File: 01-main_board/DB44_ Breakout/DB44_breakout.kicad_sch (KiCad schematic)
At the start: 7 parts, among them J1 DB44_Female, J2 Screw_Terminal_01x10 (5.08 mm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, J3 Screw_Terminal_01x10, J4 Screw_Terminal_01x10, J5 Screw_Terminal_01x10, J6 Screw_Terminal_01x02, J7 Screw_Terminal_01x02

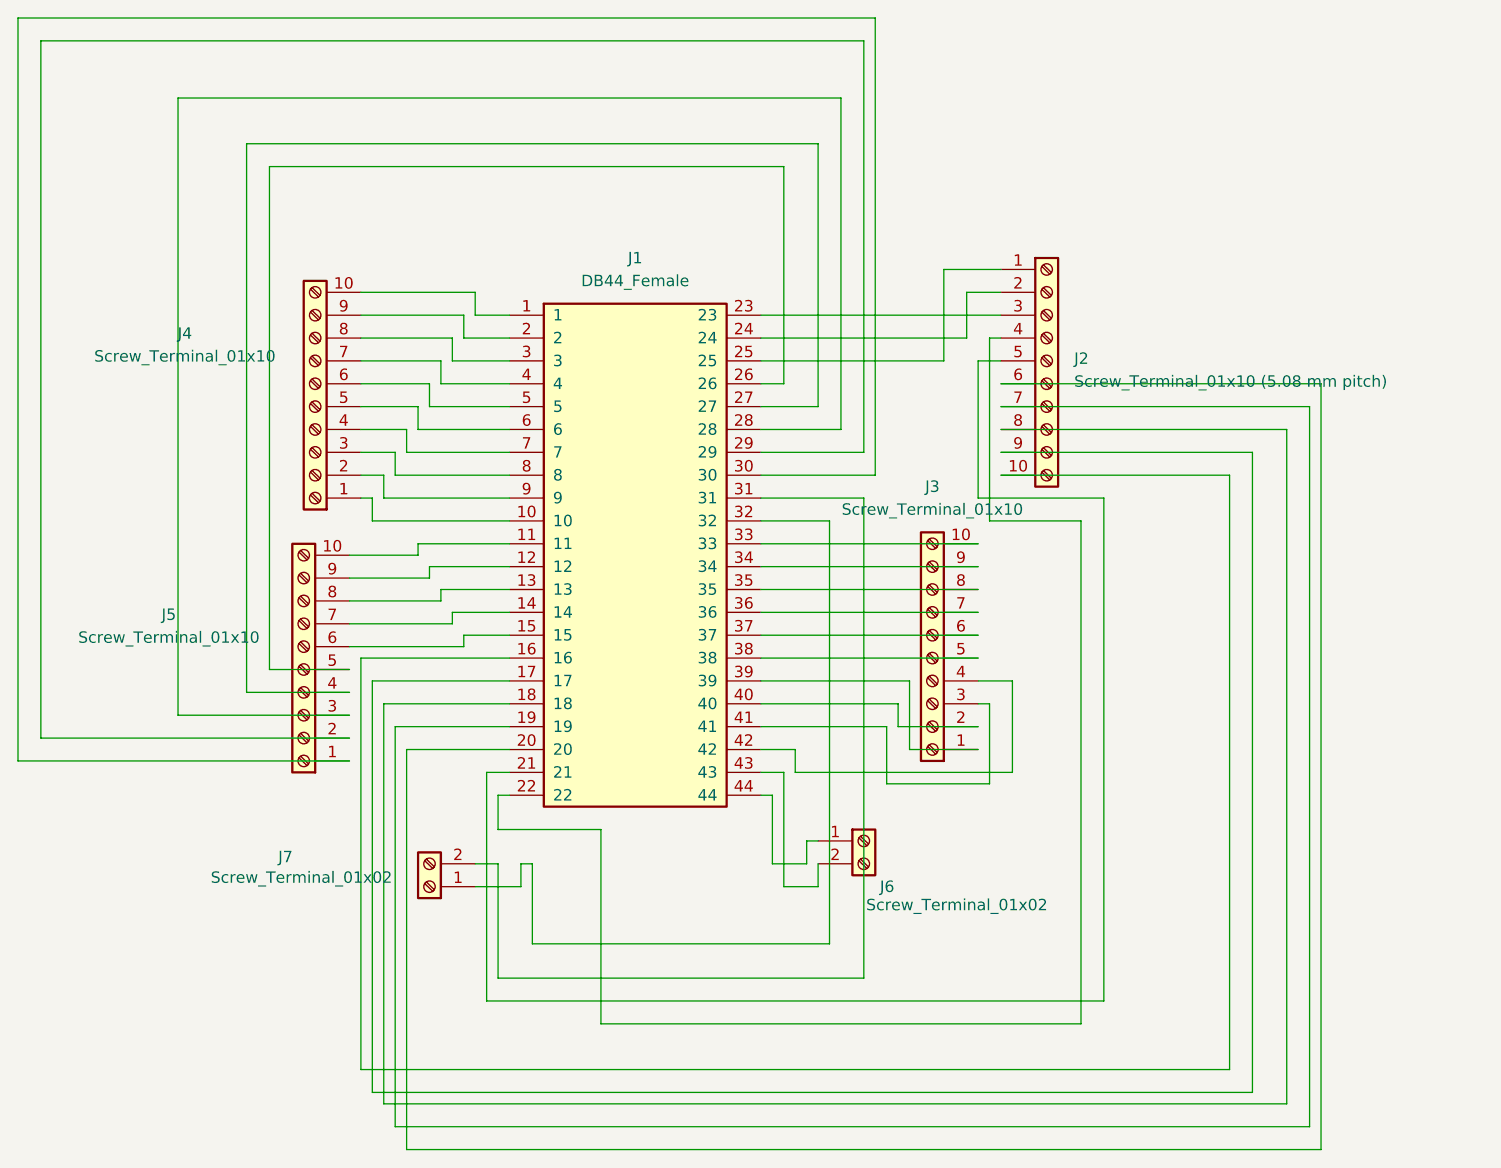
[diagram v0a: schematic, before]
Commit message: Finished DB44 board edits
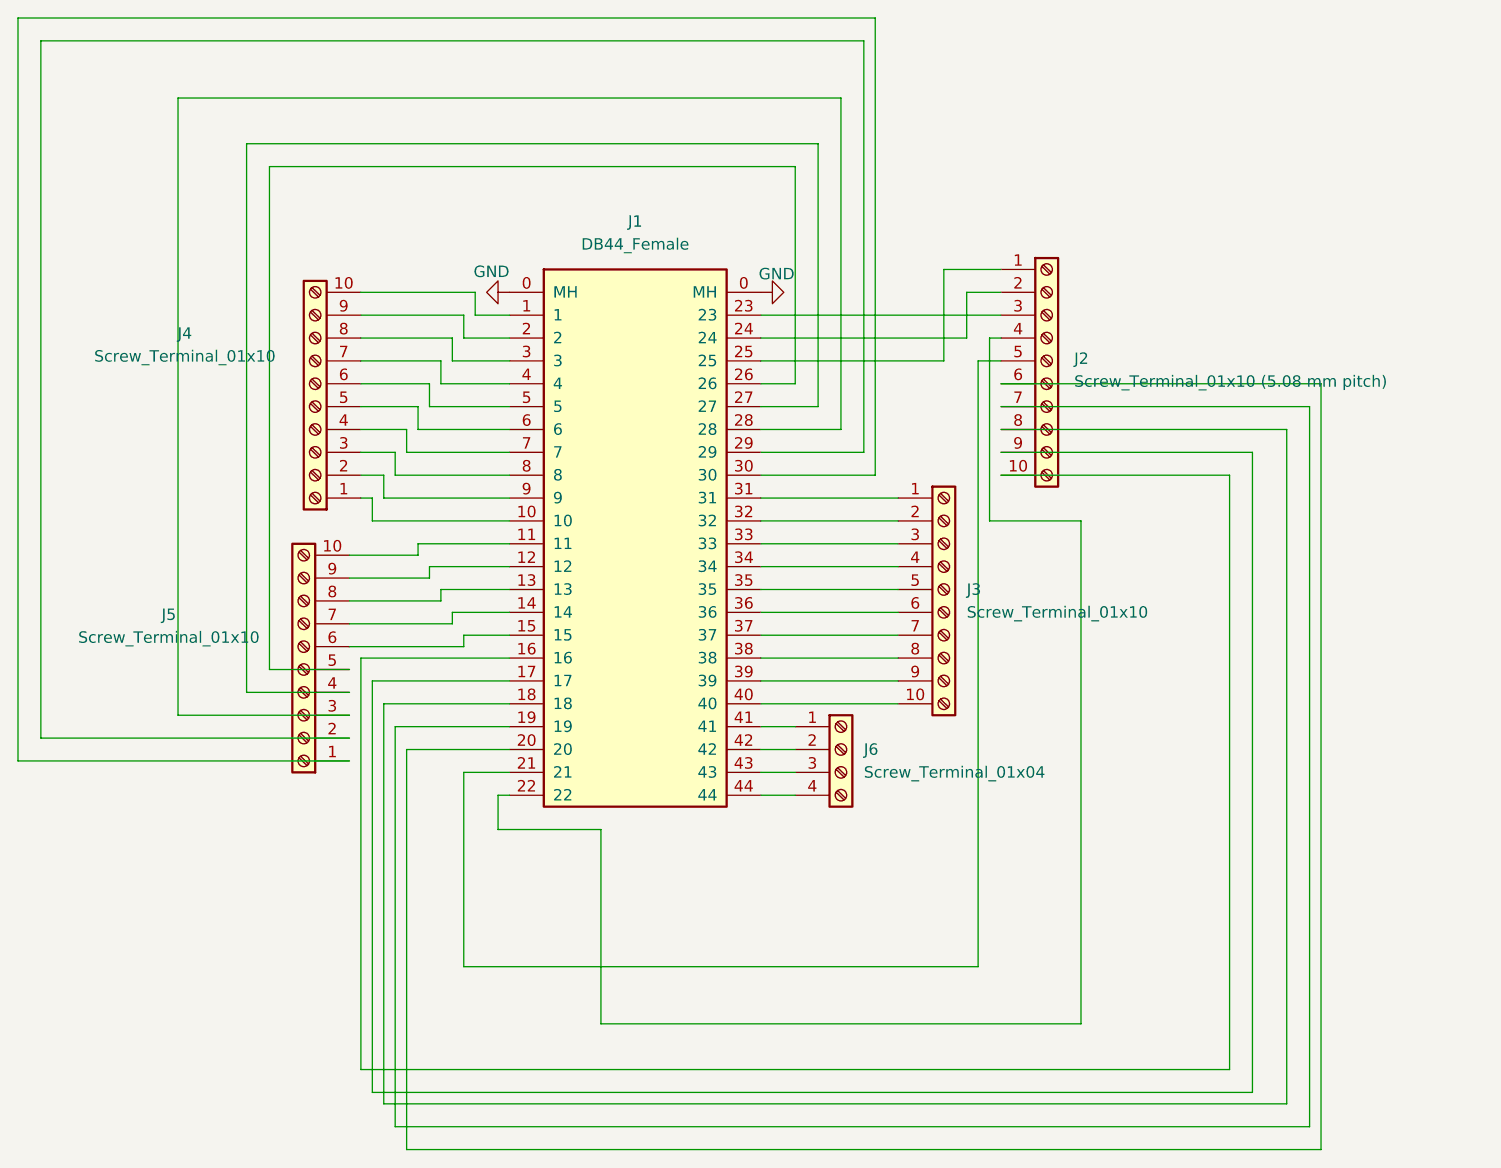
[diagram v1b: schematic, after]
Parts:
- removed J6, J7: Screw_Terminal_01x02, TerminalBlock_RND:TerminalBlock_RND_205-00232_1x02_P5.08mm_Horizontal, symbol Connector:Screw_Terminal_01x02
- added J6: Screw_Terminal_01x04, TerminalBlock_RND:TerminalBlock_RND_205-00234_1x04_P5.08mm_Horizontal, symbol Connector:Screw_Terminal_01x04
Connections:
- net at J3.1 (Pin_1): now also J1.31; no longer J1.39
- net at J3.10 (Pin_10): now also J1.40; no longer J1.33
- net at J3.2 (Pin_2): now also J1.32; no longer J1.40
- net at J3.3 (Pin_3): now also J1.33; no longer J1.41
- net at J3.4 (Pin_4): now also J1.34; no longer J1.42
- net at J3.5 (Pin_5): now also J1.35; no longer J1.38
- net at J3.6 (Pin_6): now also J1.36; no longer J1.37
- net at J3.7 (Pin_7): now also J1.37; no longer J1.36
- net at J3.8 (Pin_8): now also J1.38; no longer J1.35
- net at J3.9 (Pin_9): now also J1.39; no longer J1.34
- net at J1.44: now also J6.4 (Pin_4)
- net at J1.43: now also J6.3 (Pin_3)
- new net: J1.41, J6.1 (Pin_1)
- new net: J1.42, J6.2 (Pin_2)
- new net GND: J1.0 (MH)
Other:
- moved on the sheet: J3
